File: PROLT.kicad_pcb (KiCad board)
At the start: 4 copper layers, 80 x 80 mm, 88 parts, among them IC1 BTS4175SGA, IC2 IFX9201SGAUMA1, IC3 IFX9201SGAUMA1, J1 64334-0100, J2 USB, M1 Module:mega-mcu100/0.3, M2 Module-vr-max9924-0.1, M3 Module-power_12and5V-0.2, U1 JDY-33, U2 VNLD5160TR-E, U3 VNLD5160TR-E, U4 VNLD5160TR-E

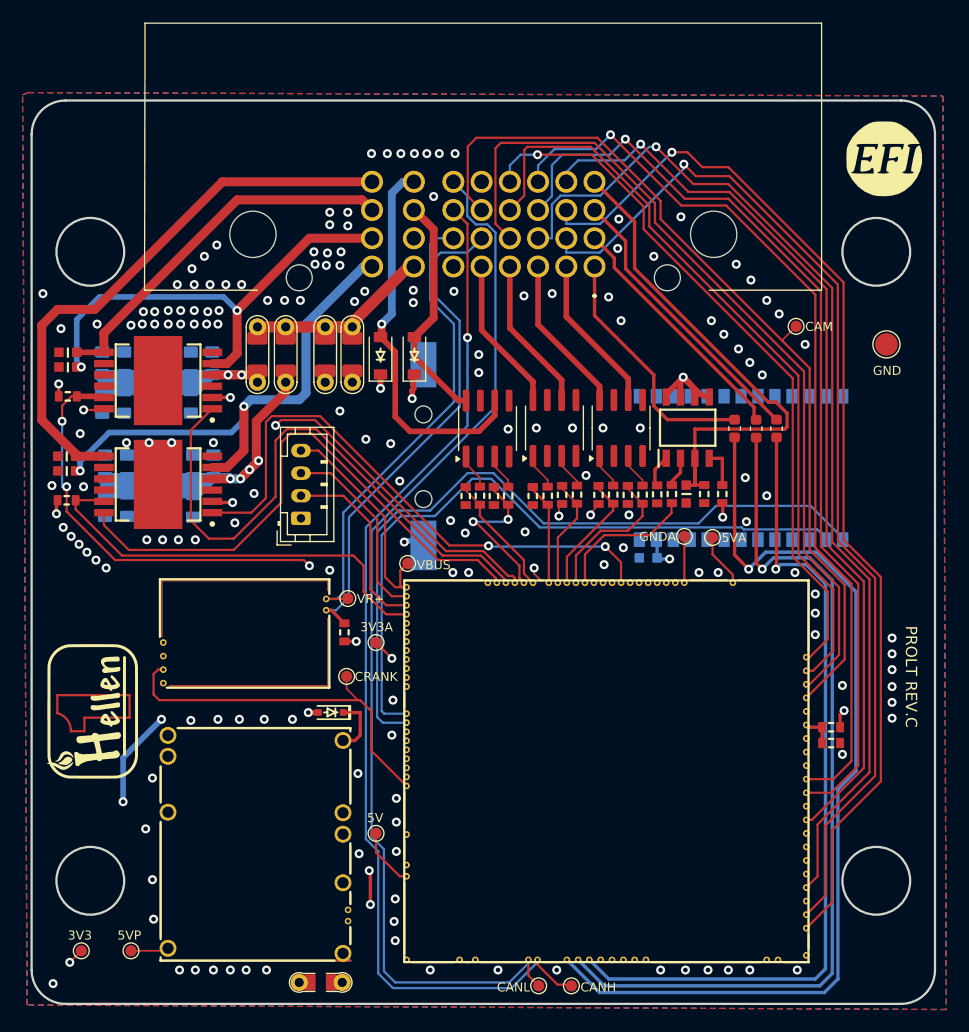
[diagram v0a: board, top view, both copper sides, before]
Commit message: Rev D
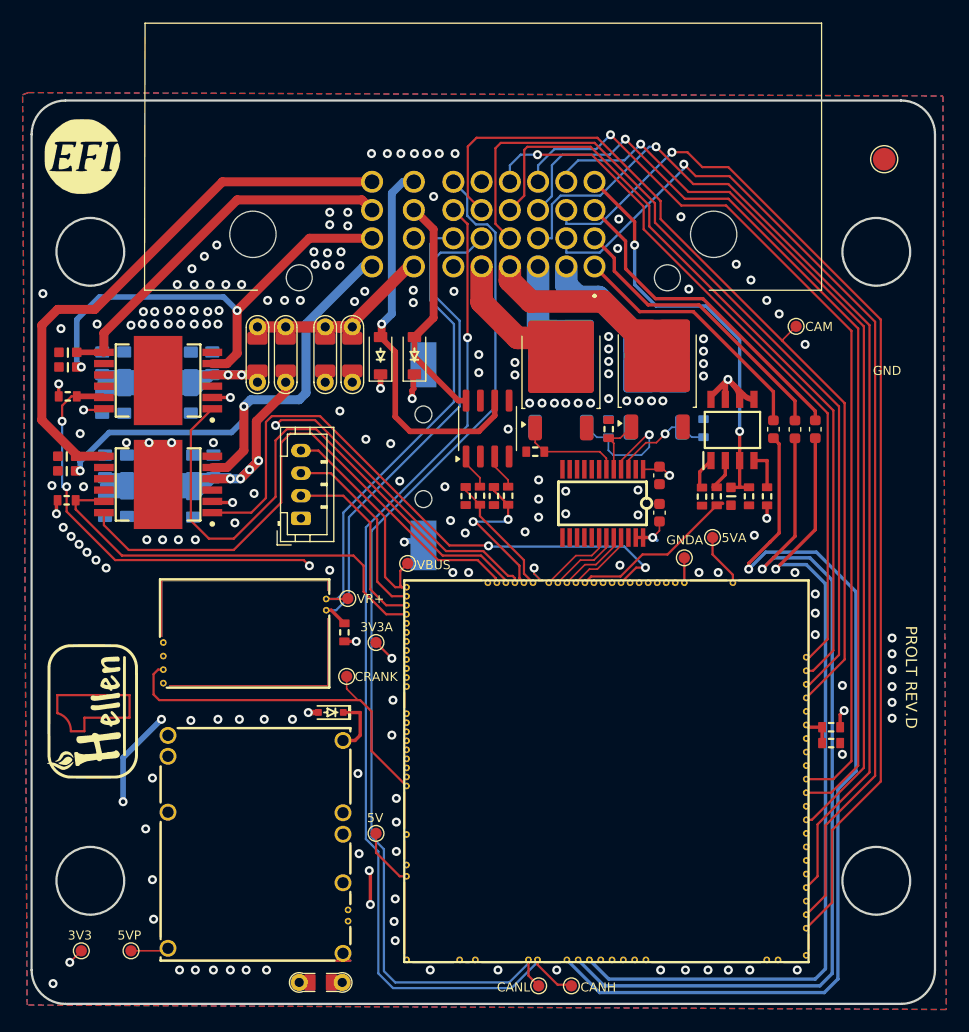
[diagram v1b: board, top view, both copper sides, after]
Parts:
- removed C28: 100n, Hellen:C0603
- removed R17, R18, R19, R20: 4.7k, Hellen:R0603
- removed U1: JDY-33, Hellen:JDY-33
- removed U3: VNLD5160TR-E, Package_SO:SOIC-8_3.9x4.9mm_P1.27mm
- added C29: 100n, Capacitor_SMD:C_0603_1608Metric, F.Cu at (162.3, 89.4)
- added C30: 100n, Capacitor_SMD:C_0603_1608Metric, F.Cu at (162.3, 92.7)
- added Q1: VND14NV04TR-E, Package_TO_SOT_SMD:TO-252-2, F.Cu at (153.6, 80.2)
- added Q2: VND14NV04TR-E, Package_TO_SOT_SMD:TO-252-2, F.Cu at (162.1, 80.1)
- added Q3: VND14NV04TR-E, Package_TO_SOT_SMD:TO-252-2, B.Cu at (153.6, 80.1)
- added Q4: VND14NV04TR-E, Package_TO_SOT_SMD:TO-252-2, B.Cu at (162.0, 80.1)
- R3, R4: moved to B.Cu
- U2: value VNLD5160TR-E -> SN74LVC4245APWR; footprint Package_SO:SOIC-8_3.9x4.9mm_P1.27mm -> EasyEda2Kicad:TSSOP-24_L7.8-W4.4-P0.65-LS6.4-BL
- moved G1 71.0 mm to (111.2, 61.2)
- moved TP13 16.4 mm to (182.2, 61.4)
- moved R4 8.93 mm to (166.2, 85.2), turned to -90 degrees
- moved U2 7.93 mm to (157.3, 91.9), turned to 180 degrees
- moved R2 7.13 mm to (157.8, 85.3), turned to -90 degrees
- moved R3 5.96 mm to (157.8, 85.2), turned to -90 degrees
- moved C1 3.97 mm to (168.6, 91.2)
- moved R5 3.97 mm to (166.1, 91.3)
- moved R6 3.97 mm to (167.4, 91.2)
- moved R7 3.97 mm to (171.8, 91.2)
- moved R8 3.97 mm to (170.2, 91.2)
- moved IC1 3.97 mm to (168.8, 85.4)
- moved R1 3.93 mm to (151.3, 87.3), turned to 0 degrees
- moved F2 3.44 mm to (174.3, 85.3)
- moved F3 3.44 mm to (176.1, 85.3)
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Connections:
- M1 pad N13: Net-(M1-UART2_TX_(PD5)) -> unconnected-(M1-UART2_TX_(PD5)-PadN13)
- M1 pad N14: Net-(M1-UART2_RX_(PD6)) -> unconnected-(M1-UART2_RX_(PD6)-PadN14)
- R1 pad 2: /INJ1_IN -> /Injectors/OUT_5V_1
- R2 pad 2: /INJ2_IN -> /Injectors/OUT_5V_2
- R3 pad 2: /INJ3_IN -> /Injectors/OUT_5V_3
- R4 pad 2: /INJ4_IN -> /Injectors/OUT_5V_4
- U2 pad 1: Net-(U2-IN1) -> +5VA
- U2 pad 2: unconnected-(U2-STATUS1-Pad2) -> GND
- U2 pad 3: Net-(U2-IN2) -> /Injectors/OUT_5V_4
- U2 pad 4: unconnected-(U2-STATUS2-Pad4) -> /Injectors/OUT_5V_3
- U2 pad 5: GND -> /Injectors/OUT_5V_2
- U2 pad 6: /INJ2_OUT -> /Injectors/OUT_5V_1
- U2 pad 7: GND -> unconnected-(U2-A5-Pad7)
- U2 pad 8: /INJ1_OUT -> unconnected-(U2-A6-Pad8)
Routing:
- net Net-(M1-UART2_RX_(PD6)): track 66.4 -> 0.00 mm
- net Net-(M1-UART2_TX_(PD5)): track 61.6 -> 0.00 mm
- net /Injectors/OUT_5V_3: track 0.00 -> 12.8 mm, vias 0 -> 1
- net /TACH: track 46.3 -> 36.6 mm, vias 0 -> 2
- net /Injectors/OUT_5V_1: track 0.00 -> 9.15 mm
- net /Injectors/OUT_5V_4: track 0.00 -> 9.03 mm, vias 0 -> 1
- net /INJ3_OUT: track 14.1 -> 6.46 mm
- net /INJ4_IN: track 13.0 -> 6.07 mm
- net +5VA: track 75.2 -> 81.3 mm, vias 0 -> 1
- net /Injectors/OUT_5V_2: track 0.00 -> 5.38 mm
- net /INJ3_IN: track 10.8 -> 6.29 mm
- net /IGN2_OUT: track 22.1 -> 26.3 mm
- net /OUT_1: track 14.1 -> 9.96 mm
- net +3.3V: track 185.2 -> 189.2 mm
- net /IGN3_OUT: track 25.2 -> 29.2 mm
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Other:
- board text added: "PROLT REV.D"
- board text removed: "PROLT REV.C"
